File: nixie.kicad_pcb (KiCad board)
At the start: 4 copper layers, 102.6 x 65.2 mm, 28 parts, among them IC1 SN74141, IC2 SN74141, IC3 SN74141, IC4 SN74141, IC5 MIC5219-5.0YM5-TR, IC6 DS3231M+TRL, J1 1984989

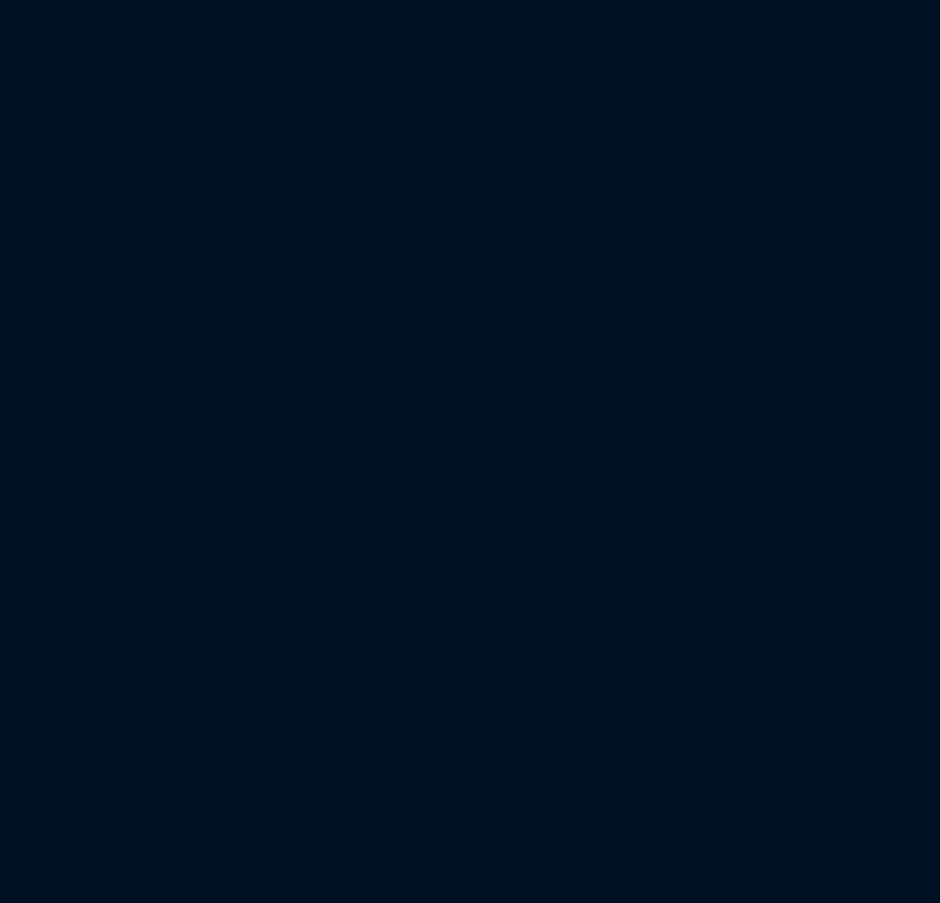
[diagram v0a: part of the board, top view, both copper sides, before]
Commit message: Adding WIP files
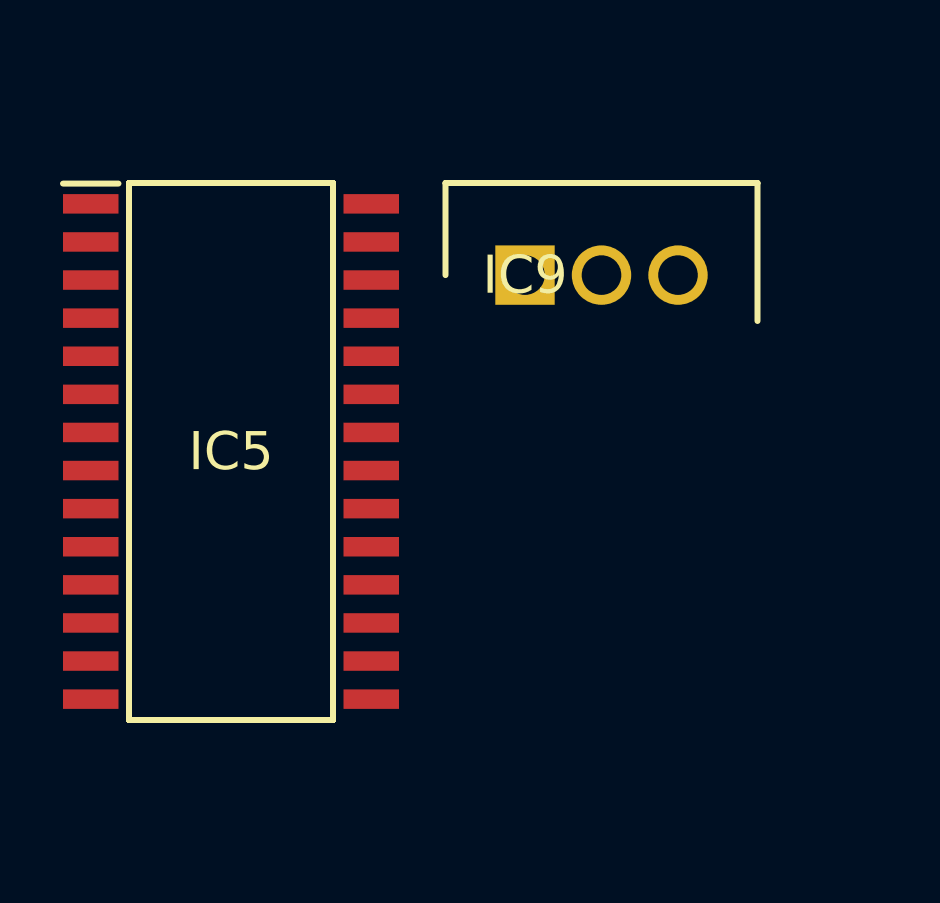
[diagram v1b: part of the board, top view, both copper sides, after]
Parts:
- added IC5: MCP23017-E_SO, L7805CV:SOIC127P1030X265-28N, F.Cu at (66.4, 111.1)
- added IC9: L7805CV, L7805CV:TO255P460X1020X2008-3P, F.Cu at (76.2, 105.2)
- N1, N2, N3, N4: value Val** -> IN-14
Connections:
- U$1 pad GP10: /A3 -> unconnected-(U$1-PadGP10)
- U$1 pad GP11: /D3 -> unconnected-(U$1-PadGP11)
- U$1 pad GP12: /B3 -> unconnected-(U$1-PadGP12)
- U$1 pad GP13: /C3 -> unconnected-(U$1-PadGP13)
- U$1 pad GP14: /A4 -> unconnected-(U$1-PadGP14)
- U$1 pad GP15: /D4 -> unconnected-(U$1-PadGP15)
- U$1 pad GP16: /C4 -> unconnected-(U$1-PadGP16)
- U$1 pad GP17: /B4 -> unconnected-(U$1-PadGP17)
- U$1 pad GP2: /A1 -> /SDA1
- U$1 pad GP3: /D1 -> /SCL1
- U$1 pad GP4: /B1 -> unconnected-(U$1-PadGP4)
- U$1 pad GP5: /C1 -> unconnected-(U$1-PadGP5)
- U$1 pad GP6: /A2 -> unconnected-(U$1-PadGP6)
- U$1 pad GP7: /D2 -> unconnected-(U$1-PadGP7)
- U$1 pad GP8: /B2 -> unconnected-(U$1-PadGP8)
- U$1 pad GP9: /C2 -> unconnected-(U$1-PadGP9)

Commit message: revert
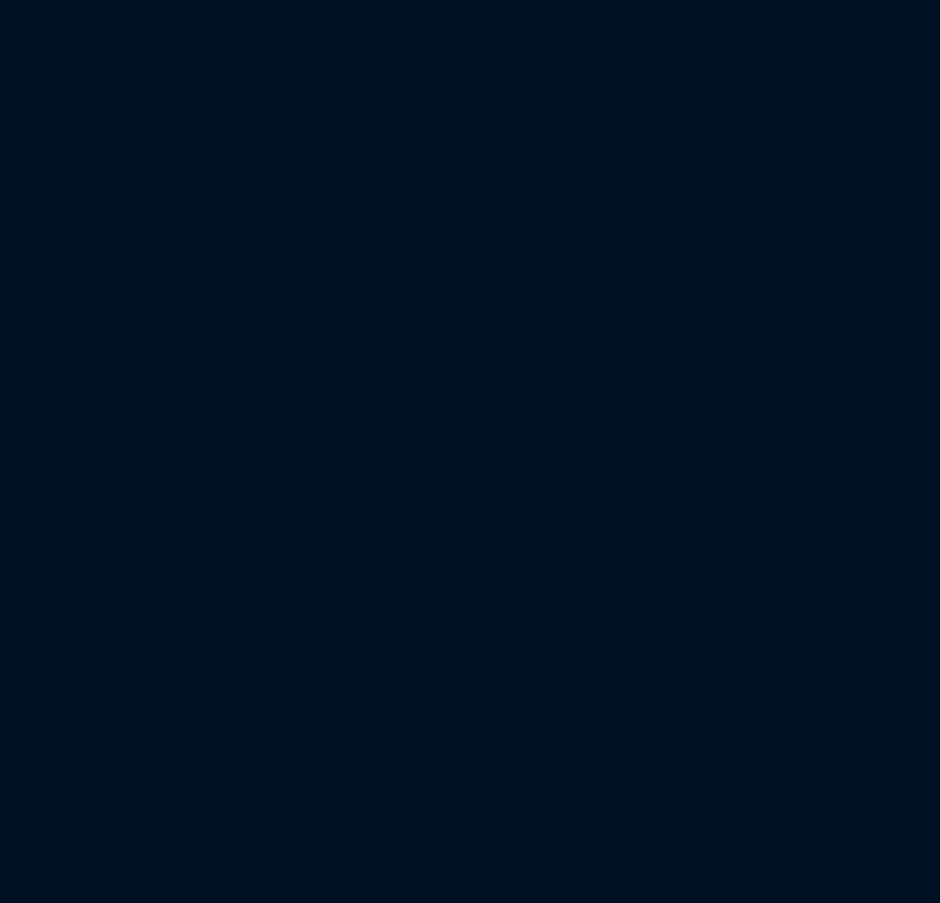
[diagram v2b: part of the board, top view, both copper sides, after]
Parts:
- removed the IC5 at (66.4, 111.1)
- removed IC9: L7805CV, L7805CV:TO255P460X1020X2008-3P
- N1, N2, N3, N4: value IN-14 -> Val**
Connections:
- U$1 pad GP10: unconnected-(U$1-PadGP10) -> /A3
- U$1 pad GP11: unconnected-(U$1-PadGP11) -> /D3
- U$1 pad GP12: unconnected-(U$1-PadGP12) -> /B3
- U$1 pad GP13: unconnected-(U$1-PadGP13) -> /C3
- U$1 pad GP14: unconnected-(U$1-PadGP14) -> /A4
- U$1 pad GP15: unconnected-(U$1-PadGP15) -> /D4
- U$1 pad GP16: unconnected-(U$1-PadGP16) -> /C4
- U$1 pad GP17: unconnected-(U$1-PadGP17) -> /B4
- U$1 pad GP2: /SDA1 -> /A1
- U$1 pad GP3: /SCL1 -> /D1
- U$1 pad GP4: unconnected-(U$1-PadGP4) -> /B1
- U$1 pad GP5: unconnected-(U$1-PadGP5) -> /C1
- U$1 pad GP6: unconnected-(U$1-PadGP6) -> /A2
- U$1 pad GP7: unconnected-(U$1-PadGP7) -> /D2
- U$1 pad GP8: unconnected-(U$1-PadGP8) -> /B2
- U$1 pad GP9: unconnected-(U$1-PadGP9) -> /C2
